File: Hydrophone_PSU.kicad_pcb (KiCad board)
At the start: 2 copper layers, 50.1 x 158.5 mm, 27 parts, among them J1 Screw_Terminal_01x02, J2 Screw_Terminal_01x03, U1 LT8471IFE_PBF

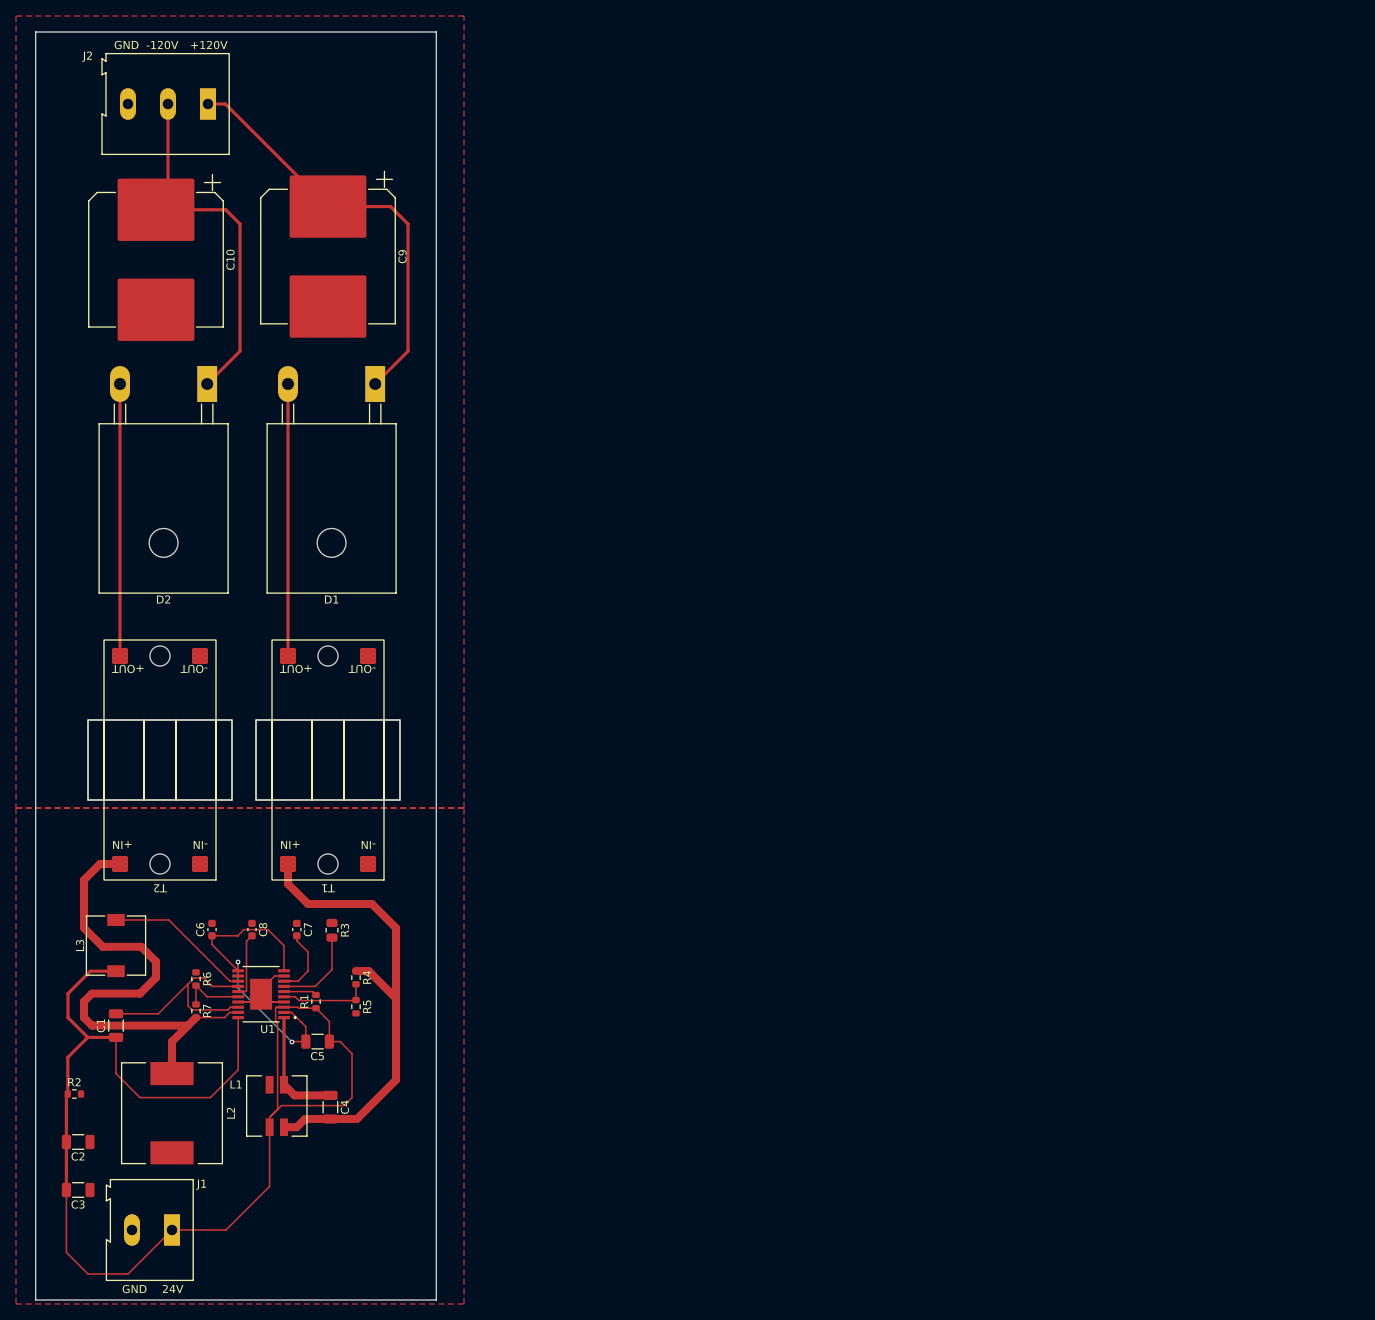
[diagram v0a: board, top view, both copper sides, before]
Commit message: poprawki Tadeusz
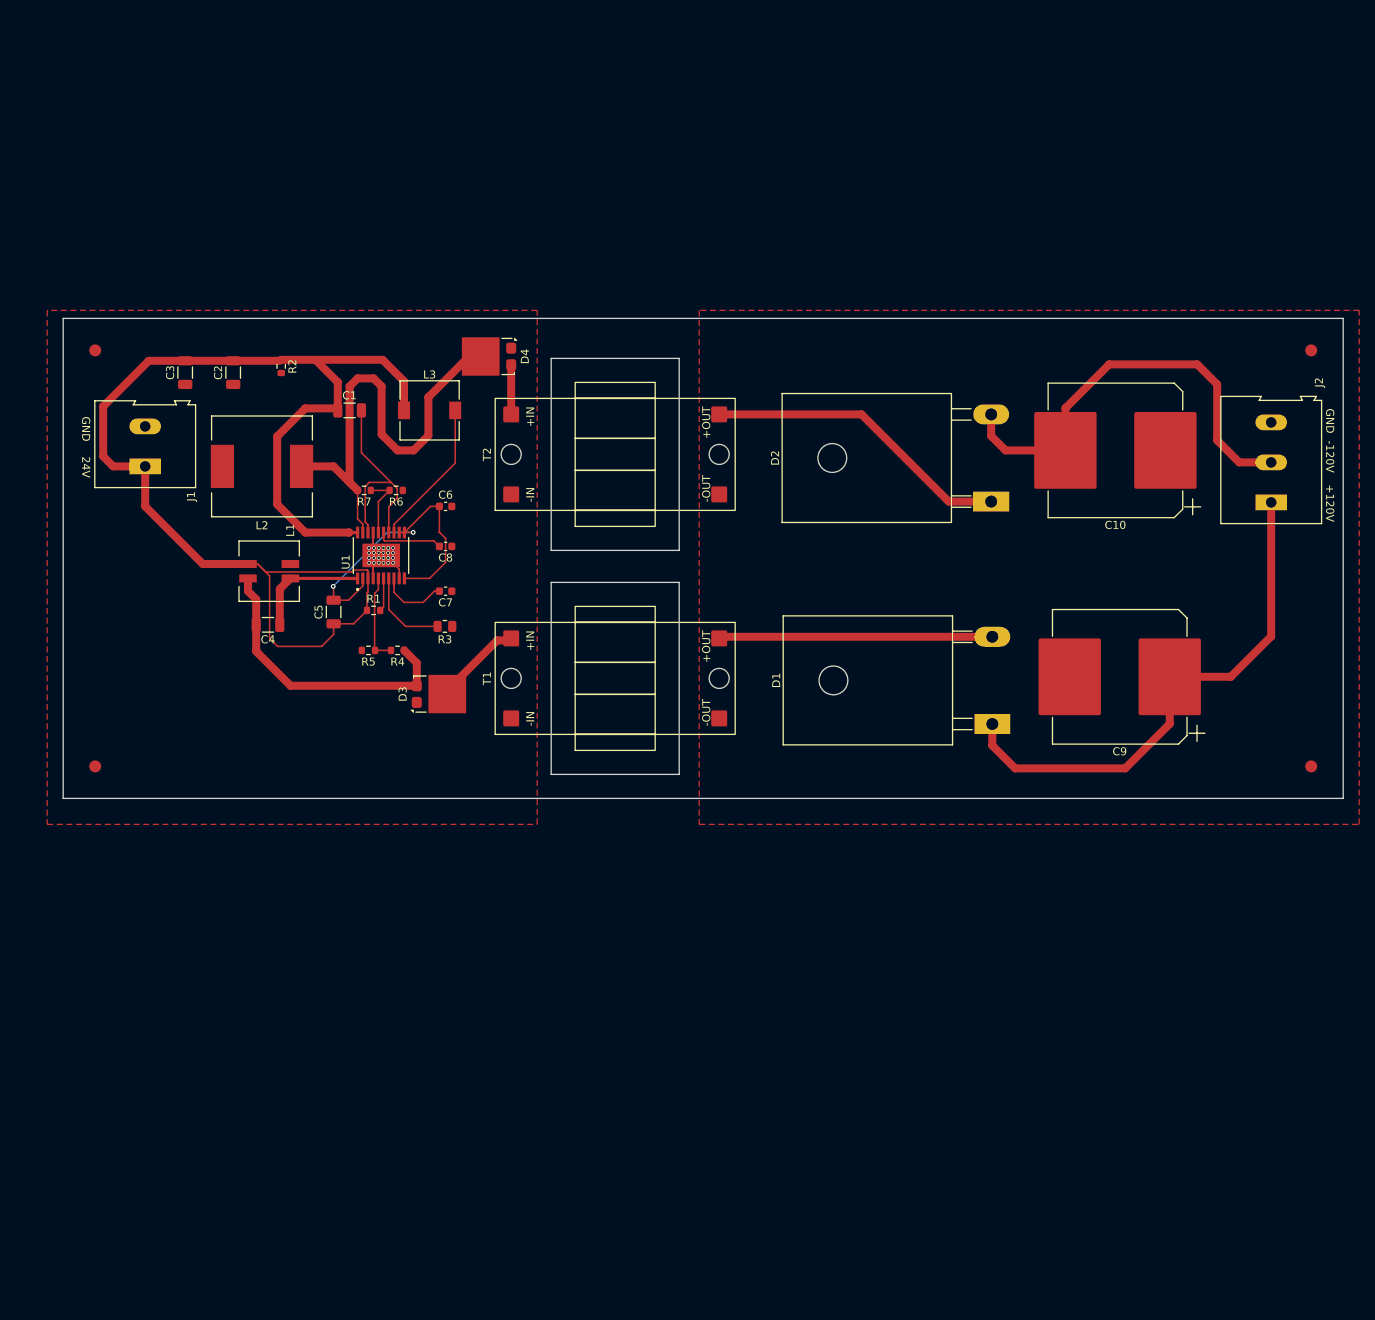
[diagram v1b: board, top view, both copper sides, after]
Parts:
- added D3: V10P10, Package_TO_SOT_SMD:TO-277A, F.Cu at (82.9, 99.8)
- added D4: V10P10, Package_TO_SOT_SMD:TO-277A, F.Cu at (89.1, 57.6)
- added REF**: Fiducial_1.5mm_Mask3mm, Fiducial:Fiducial_1.5mm_Mask3mm, F.Cu at (191.9, 56.8)
- added REF**: Fiducial_1.5mm_Mask3mm, Fiducial:Fiducial_1.5mm_Mask3mm, F.Cu at (39.9, 56.8)
- added REF**: Fiducial_1.5mm_Mask3mm, Fiducial:Fiducial_1.5mm_Mask3mm, F.Cu at (39.9, 108.8)
- added REF**: Fiducial_1.5mm_Mask3mm, Fiducial:Fiducial_1.5mm_Mask3mm, F.Cu at (191.9, 108.8)
- moved J2 141.9 mm to (186.9, 75.8), turned to 90 degrees
- moved C10 122.3 mm to (167.4, 69.3), turned to 180 degrees
- moved C9 112.0 mm to (168.0, 97.6), turned to 180 degrees
- moved C3 103.0 mm to (51.1, 59.6), turned to 90 degrees
- moved D2 99.1 mm to (151.9, 75.7), turned to 90 degrees
- moved C2 98.1 mm to (57.1, 59.6), turned to 90 degrees
- moved J1 95.5 mm to (46.1, 71.3), turned to 90 degrees
- moved R2 94.6 mm to (63.1, 58.8), turned to -90 degrees
- moved D1 88.1 mm to (152.0, 103.5), turned to 90 degrees
- moved C1 82.3 mm to (71.7, 64.3), turned to 0 degrees
- moved L2 81.6 mm to (60.8, 71.3), turned to 180 degrees
- moved T2 77.6 mm to (122.9, 69.8), turned to 90 degrees
- moved L3 77.5 mm to (81.7, 64.3), turned to 0 degrees
- moved R7 68.4 mm to (73.5, 74.3), turned to 180 degrees
- moved L1 66.9 mm to (61.6, 84.4), turned to 90 degrees
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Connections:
- C10 pad 1: HV- -> GND
- C10 pad 2: GND -> HV-
- C4 pad 2: +20VSQW -> Net-(C4-Pad2)
- D2 pad 1: HV- -> Net-(D2-K)
- D2 pad 2: Net-(D2-A) -> HV-
- L1 pad 2: +20VSQW -> Net-(C4-Pad2)
- L2 pad 1: -20VSQW -> Net-(D4-K)
- R4 pad 1: +20VSQW -> Net-(C4-Pad2)
- R7 pad 2: -20VSQW -> Net-(D4-K)
- T2 pad 4: Net-(D2-A) -> Net-(D2-K)
- U1 pad 19: -20VSQW -> Net-(D4-K)
- U1 pad 21: GND -> Net-(U1-E1)
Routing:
- net Net-(D4-K): track 0.00 -> 57.5 mm
- net -20VSQW: track 63.5 -> 6.20 mm
- net +20VSQW: track 60.1 -> 11.0 mm
- net Net-(D2-K): track 0.00 -> 38.5 mm
- net Net-(C4-Pad2): track 0.00 -> 36.5 mm
- net Net-(D2-A): track 34.0 -> 0.00 mm
- net HV+: track 52.9 -> 65.8 mm
- net HV-: track 46.8 -> 55.2 mm
- net GND: track 17.2 -> 19.3 mm
- net C2: track 158.7 -> 160.0 mm
- net (no net): vias 0 -> 24
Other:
- board size 50.1 x 158.5 mm -> 160 x 60 mm
